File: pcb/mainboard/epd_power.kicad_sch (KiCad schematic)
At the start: 80 parts, among them Q1 AO3401A, Q2 S8050, Q6 AO3400A, Q7 AO3401A, Q8 AO3401A, U10 LGS5148, U11 LM321, U21 INA3221, U22 INA3221, U6 MT9700, U7 MT3608(SOT23-6), U8 MT3608(SOT23-6), U9 LGS5148

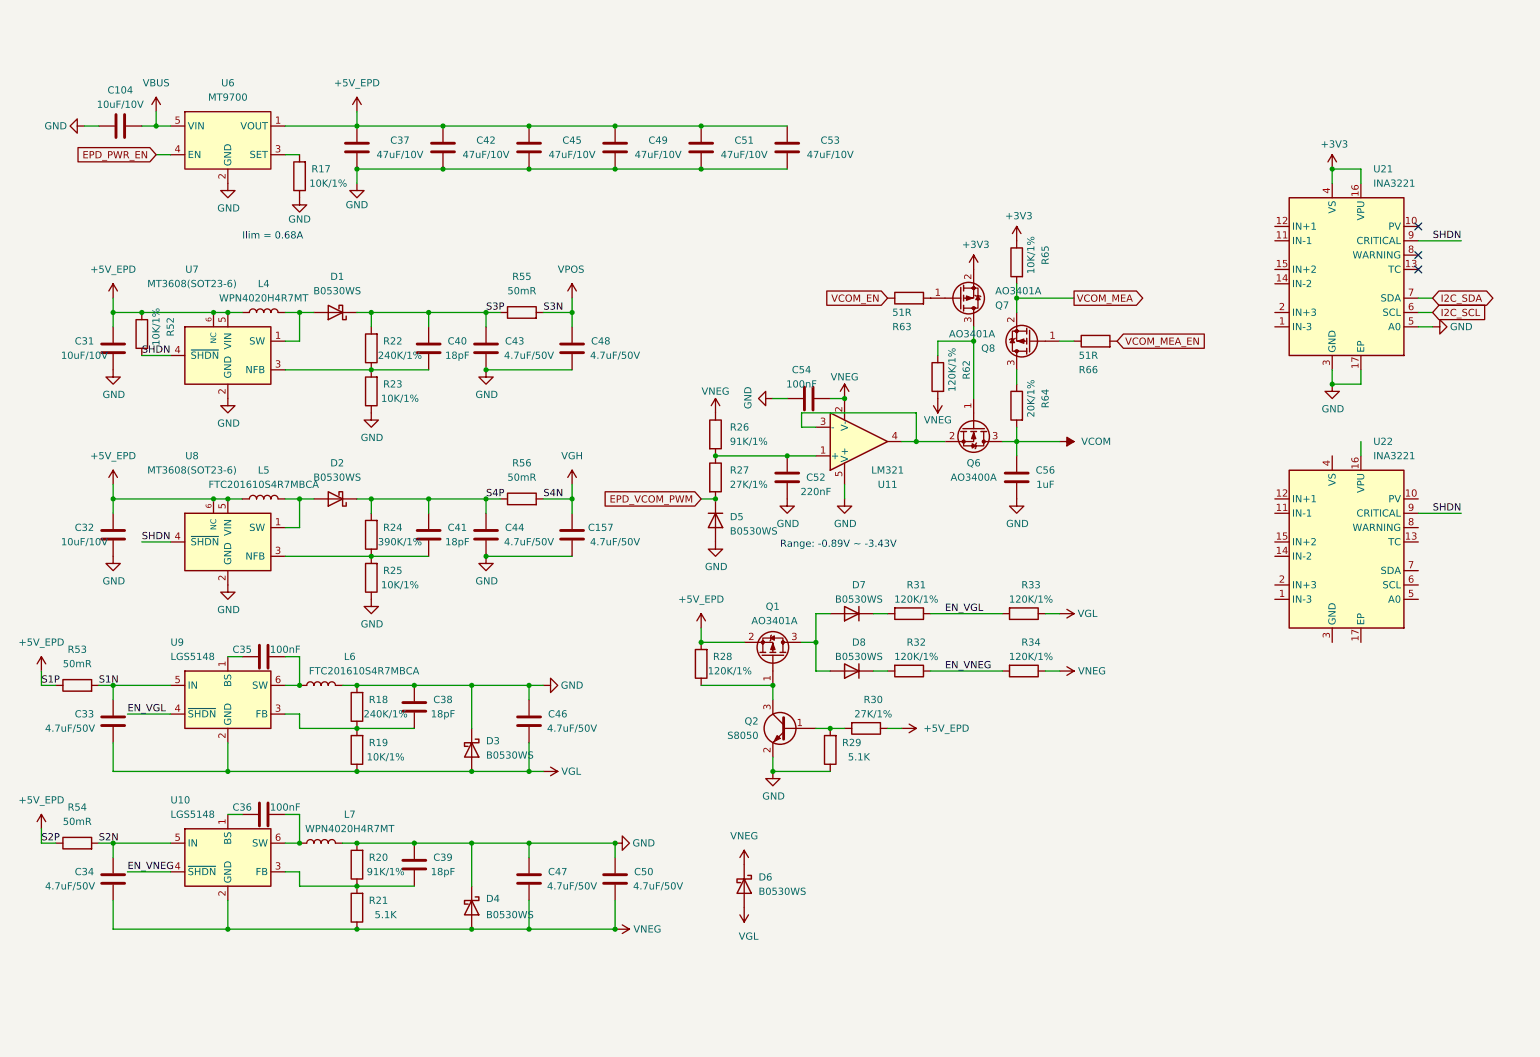
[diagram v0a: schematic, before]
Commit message: PCB r0p9
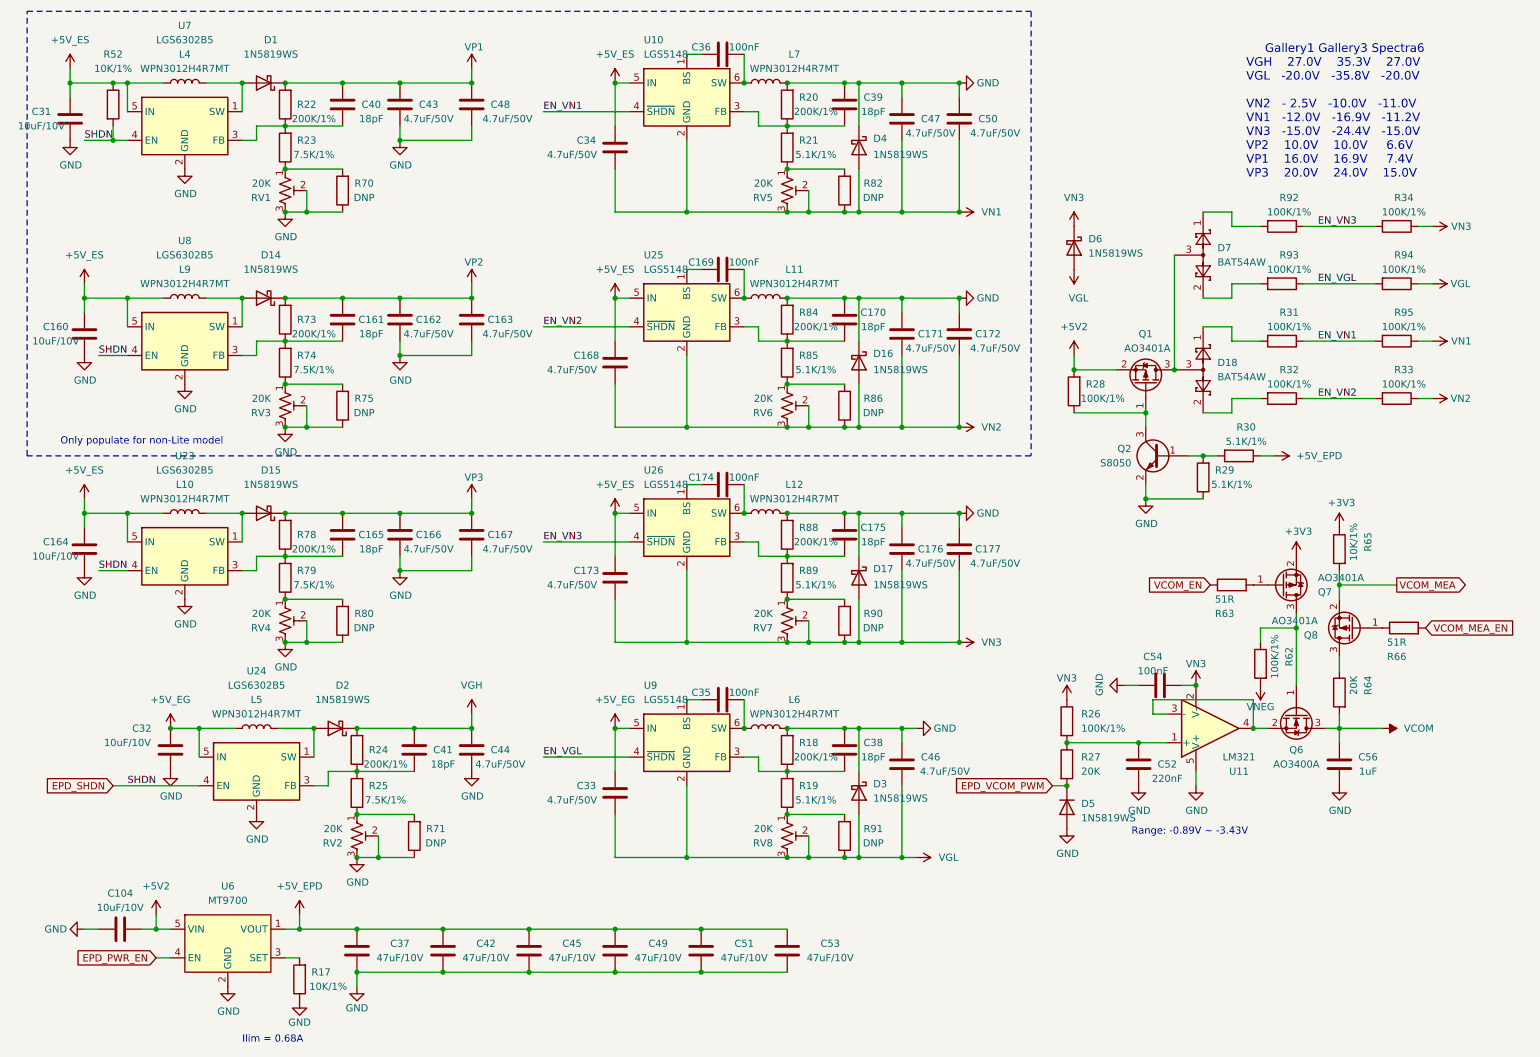
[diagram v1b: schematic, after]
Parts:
- removed C157: 4.7uF/50V, Capacitor_SMD:C_0805_2012Metric, symbol Device:C
- removed D7, D8: B0530WS, Diode_SMD:D_SOD-323, symbol Device:D
- removed R53, R54, R55, R56: 50mR, Resistor_SMD:R_0805_2012Metric, symbol Device:R
- removed U21, U22: INA3221, Package_DFN_QFN:Texas_RGV0016A_VQFN-16-1EP_4x4mm_P0.65mm_EP2.1x2.1mm, symbol Power_Management:INA3221
- removed U7, U8: MT3608(SOT23-6), Package_TO_SOT_SMD:SOT-23-6, symbol symbols:MT3608(SOT23-6)
- added C160, C164: 10uF/10V, Capacitor_SMD:C_0603_1608Metric, symbol Device:C
- added C161, C165, C170, C175: 18pF, Capacitor_SMD:C_0402_1005Metric, symbol Device:C
- added C162, C163, C166, C167, C168, C171, C172, C173, C176, C177: 4.7uF/50V, Capacitor_SMD:C_0805_2012Metric, symbol Device:C
- added C169, C174: 100nF, Capacitor_SMD:C_0402_1005Metric, symbol Device:C
- added D14, D15, D16, D17: 1N5819WS, Diode_SMD:D_SOD-323, symbol Diode:1N5819WS
- added D18, D7: BAT54AW, Package_TO_SOT_SMD:SOT-323_SC-70, symbol Diode:BAT54AW
- added L10, L11, L12, L9: WPN3012H4R7MT, Inductor_SMD:L_Changjiang_FNR3012S, symbol Device:L
- added R70, R71, R75, R80, R82, R86, R90, R91: DNP, Resistor_SMD:R_0402_1005Metric, symbol Device:R
- added R73, R78, R84, R88: 200K/1%, Resistor_SMD:R_0402_1005Metric, symbol Device:R
- added R74, R79: 7.5K/1%, Resistor_SMD:R_0402_1005Metric, symbol Device:R
- added R85, R89: 5.1K/1%, Resistor_SMD:R_0402_1005Metric, symbol Device:R
- added R92, R93, R94, R95: 100K/1%, Resistor_SMD:R_0402_1005Metric, symbol Device:R
- added RV1, RV2, RV3, RV4, RV5, RV6, RV7, RV8: 20K, footprints:Potentiometer_Bourns_TC33X_Vertical, symbol Device:R_Potentiometer_Trim_US
- added U23, U24, U7, U8: LGS6302B5, Package_TO_SOT_SMD:SOT-23-5, symbol Regulator_Switching:LGS6302B5
- added U25, U26: LGS5148, Package_TO_SOT_SMD:TSOT-23-6, symbol symbols:SY8120
- C104, C31, C32: footprint Capacitor_SMD:C_0805_2012Metric -> Capacitor_SMD:C_0603_1608Metric
- C37, C42, C45, C49, C51, C53: footprint Capacitor_SMD:C_1206_3216Metric -> Capacitor_SMD:C_0805_2012Metric
- D1, D2, D3, D4, D5, D6: value B0530WS -> 1N5819WS
- L4, L7: value WPN4020H4R7MT -> WPN3012H4R7MT; footprint Inductor_SMD:L_Changjiang_FNR4020S -> Inductor_SMD:L_Changjiang_FNR3012S
- L5, L6: value FTC201610S4R7MBCA -> WPN3012H4R7MT; footprint Inductor_SMD:L_Murata_DFE201610P -> Inductor_SMD:L_Changjiang_FNR3012S
- R18, R22: value 240K/1% -> 200K/1%
- R19: value 10K/1% -> 5.1K/1%
- R20: value 91K/1% -> 200K/1%
- R21, R29: value 5.1K -> 5.1K/1%
- R23, R25: value 10K/1% -> 7.5K/1%
- R24: value 390K/1% -> 200K/1%
- R26: value 91K/1% -> 100K/1%
- R27: value 27K/1% -> 20K
- R28, R31, R32, R33, R34, R62: value 120K/1% -> 100K/1%
- R30: value 27K/1% -> 5.1K/1%
- R64: value 20K/1% -> 20K
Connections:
- net S4P is gone; now on net VGH: C41.2, C44.2, D2.1 (K), R24.2
- net VPOS is gone; now on net VP1: C48.2
- net +5V_EPD: no longer C31.2, C32.2, L4.1, L5.1, Q1.2 (S), R28.2, R52.1
- net EN_VGL: now also R93.1, R94.2; no longer R31.1, R33.2
- net GND: now also C160.1, C162.1, C163.1, C164.1, C166.1, C167.1, C170.2, C171.2, C172.2, C175.2, C176.2, C177.2, D16.1 (K), D17.1 (K), L11.2, L12.2, R70.1, R71.1, R75.1, R80.1, R84.2, R88.2, RV1.2, RV1.3, RV2.2, RV2.3, RV3.2, RV3.3, RV4.2, RV4.3, U23.2 (GND), U24.2 (GND), U7.2 (GND), U8.2 (GND); no longer R23.1, R25.1
- net VGL: now also R91.1, R94.1, RV8.2, RV8.3; no longer R19.1, R33.1
- net VNEG: no longer C34.1, C47.1, C50.1, C54.2, D4.2 (A), D6.1 (K), R21.1, R26.1, R34.1, U10.2 (GND), U11.2 (V-)
- net at D1.2 (A), L4.2: now also U7.1 (SW)
- net at R32.2: now also D18.2
- net at C40.1, R22.1, R23.2: now also U7.3 (FB)
- net at R31.2: now also D18.1
- net at Q1.3 (D): now also D18.3, D7.3
- net at C41.1, R24.1, R25.2: now also U24.3 (FB)
- net at D2.2 (A), L5.2: now also U24.1 (SW)
- removed net EN_VNEG: R32.1, R34.2, U10.4 (~{SHDN})
- net S1N renamed +5V_EG
- net +5V_EG: now also C32.2, L5.1, U24.5 (IN)
- net S2N renamed +5V_ES
- net +5V_ES: now also C31.2, L4.1, R52.1, C160.2, C164.2, C168.2, C173.2, L10.1, L9.1, U23.5 (IN), U25.5 (IN), U26.5 (IN), U7.5 (IN), U8.5 (IN)
- net S3P renamed VP1
- net SHDN renamed EPD_SHDN
- net EPD_SHDN: now also U23.4 (EN), U24.4 (EN), U7.4 (EN), U8.4 (EN)
- net VBUS renamed +5V2
- net +5V2: now also Q1.2 (S), R28.2
- new net: C169.1, L11.1, U25.6 (SW)
- new net: D7.2, R93.2
- new net: R74.1, R75.2, RV3.1
- new net: D14.2 (A), L9.2, U8.1 (SW)
- new net: C161.1, R73.1, R74.2, U8.3 (FB)
- new net: R85.1, R86.2, RV6.1
- new net: C170.1, R84.1, R85.2, U25.3 (FB)
- new net: R23.1, R70.2, RV1.1
- new net: C174.2, U26.1 (BS)
- new net: C175.1, R88.1, R89.2, U26.3 (FB)
- new net: C174.1, L12.1, U26.6 (SW)
- new net: R79.1, R80.2, RV4.1
- new net: R21.1, R82.2, RV5.1
- new net: R89.1, R90.2, RV7.1
- new net: D15.2 (A), L10.2, U23.1 (SW)
- new net: D7.1, R92.2
- new net: R25.1, R71.2, RV2.1
- new net: R19.1, R91.2, RV8.1
- new net: C165.1, R78.1, R79.2, U23.3 (FB)
- new net: C169.2, U25.1 (BS)
- new net EN_VN1: R31.1, R95.2, U10.4 (~{SHDN})
- new net EN_VN2: R32.1, R33.2, U25.4 (~{SHDN})
- new net EN_VN3: R34.2, R92.1, U26.4 (~{SHDN})
- new net VN1: C34.1, C47.1, C50.1, D4.2 (A), R82.1, R95.1, RV5.2, RV5.3, U10.2 (GND)
- new net VN2: C168.1, C171.1, C172.1, D16.2 (A), R33.1, R86.1, RV6.2, RV6.3, U25.2 (GND)
- new net VN3: C173.1, C176.1, C177.1, C54.2, D17.2 (A), D6.1 (K), R26.1, R34.1, R90.1, RV7.2, RV7.3, U11.2 (V-), U26.2 (GND)
- new net VP2: C161.2, C162.2, C163.2, D14.1 (K), R73.2
- new net VP3: C165.2, C166.2, C167.2, D15.1 (K), R78.2
- no-connect marks 3 -> 0
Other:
- note added: "Gallery1 Gallery3 Spectra6 VGH 27.0V 35.3V 27.0V VGL -20.0V -35.8V -20.0V VN2 - 2.5V -10.0V -11.0V VN1 -12.0V -16.9V -11.2V VN3 -15.0V -24.4V -15.0V VP2 10.0V 10.0V 6.6V VP1 16.0V 16.9V 7.4V VP3 20.0V 24.0V 15.0V"
- note added: "Only populate for non-Lite model"
- moved on the sheet: C104, C31, C32, C33, C34, C35, C36, C37, C38, C39, C40, C41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
